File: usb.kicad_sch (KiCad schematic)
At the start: 20 parts, among them J2 TYPE-C 16PIN 2MD(073), U3 TPS25200DRVT, U4 USBLC6-2P6, U5 USBLC6-2P6

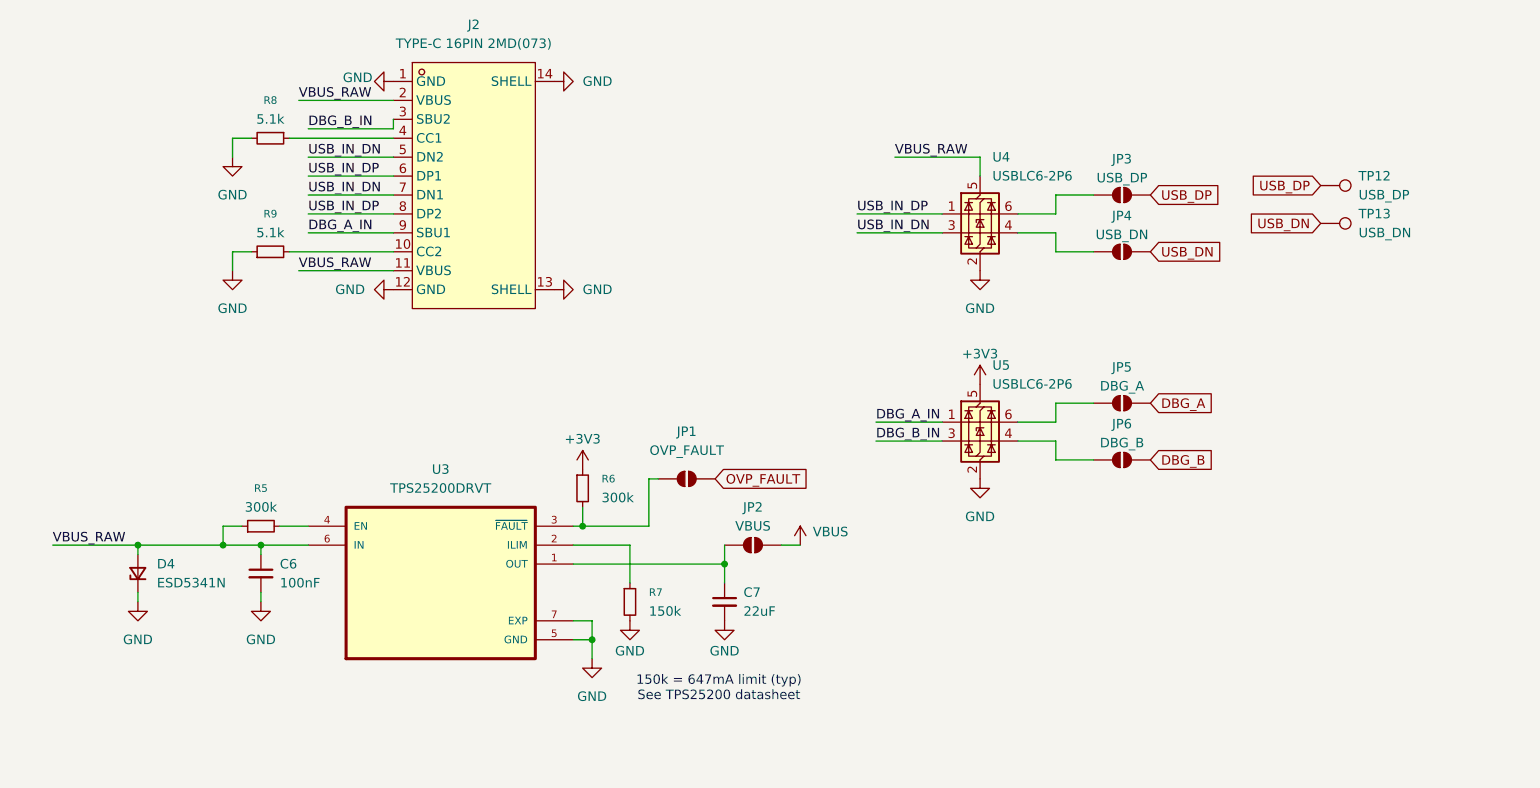
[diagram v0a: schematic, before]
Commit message: huge progress on bentoboard, schematic fixes
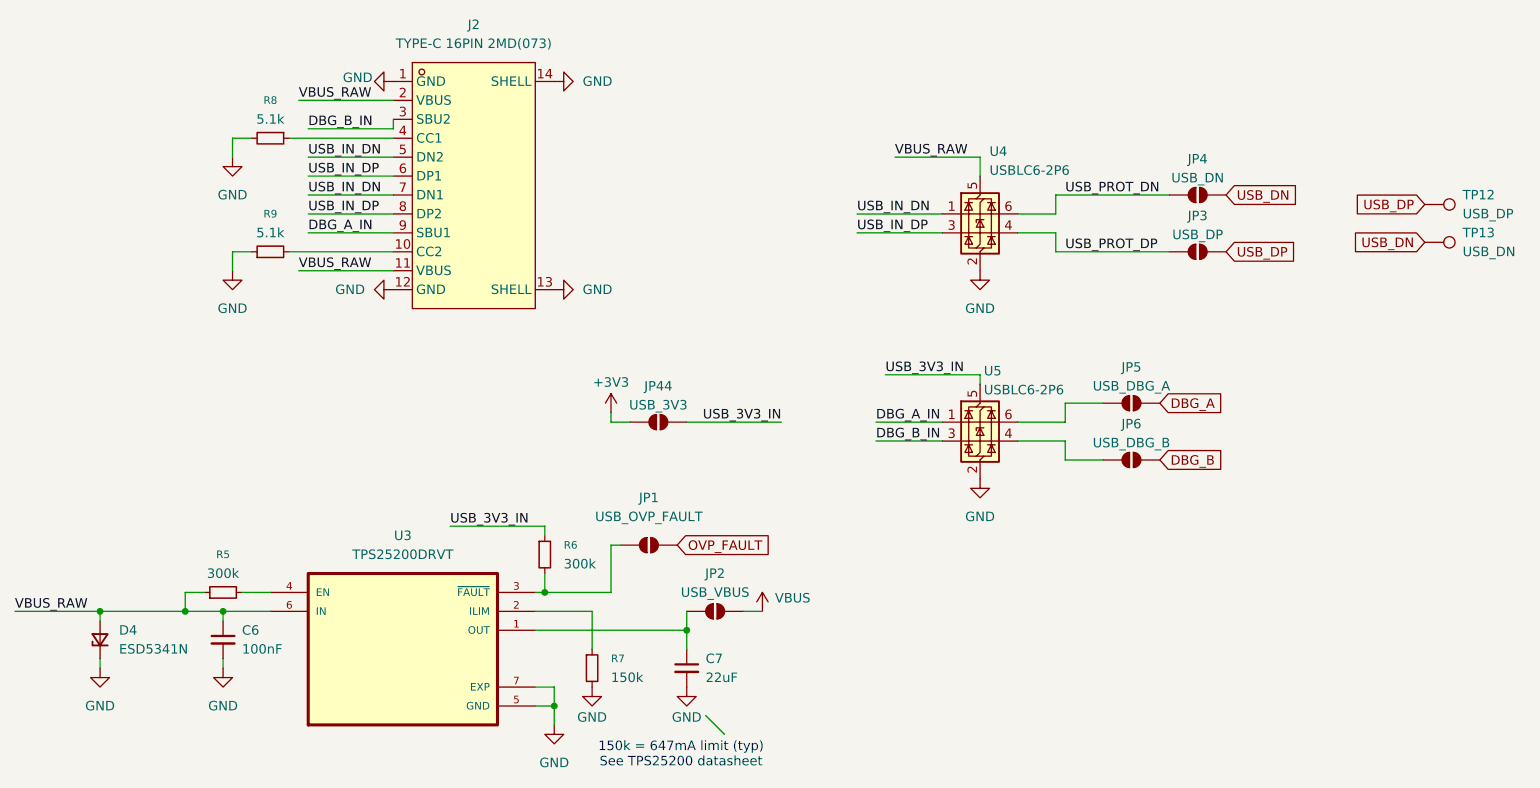
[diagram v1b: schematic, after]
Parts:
- added JP44: USB_3V3, Jumper:SolderJumper-2_P1.3mm_Open_Pad1.0x1.5mm, symbol Jumper:SolderJumper_2_Open
- JP1: value OVP_FAULT -> USB_OVP_FAULT
- JP2: value VBUS -> USB_VBUS
- JP5: value DBG_A -> USB_DBG_A
- JP6: value DBG_B -> USB_DBG_B
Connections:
- net +3V3: now also JP44.1 (A); no longer R6.1, U5.5 (VBUS)
- net USB_IN_DN: now also U4.1 (I/O1); no longer U4.3 (I/O2)
- net USB_IN_DP: now also U4.3 (I/O2); no longer U4.1 (I/O1)
- net USB_PROT_DN: now reaches JP4.1 (A)
- net USB_PROT_DN: now also U4.6 (I/O1); no longer U4.4 (I/O2)
- net USB_PROT_DP: now reaches JP3.1 (A)
- net USB_PROT_DP: now also U4.4 (I/O2); no longer U4.6 (I/O1)
- new net USB_3V3_IN: JP44.2 (B), R6.1, U5.5 (VBUS)
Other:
- moved on the sheet: C6, C7, D4, JP1, JP2, JP3, JP4, JP5, JP6, R5, R6, R7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
